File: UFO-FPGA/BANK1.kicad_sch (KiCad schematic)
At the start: 7 parts, among them U1 ICE40HX8K-BG121

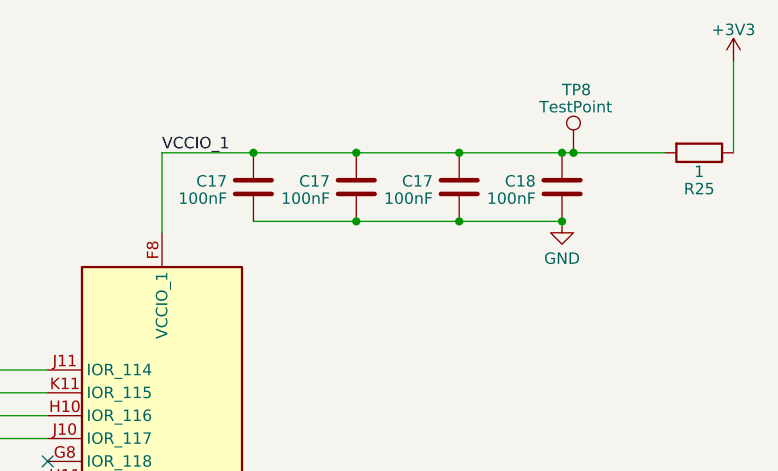
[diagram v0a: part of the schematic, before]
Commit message: PCB
many pcb changes
-started routing
-added vias
-power planes
-ground planes
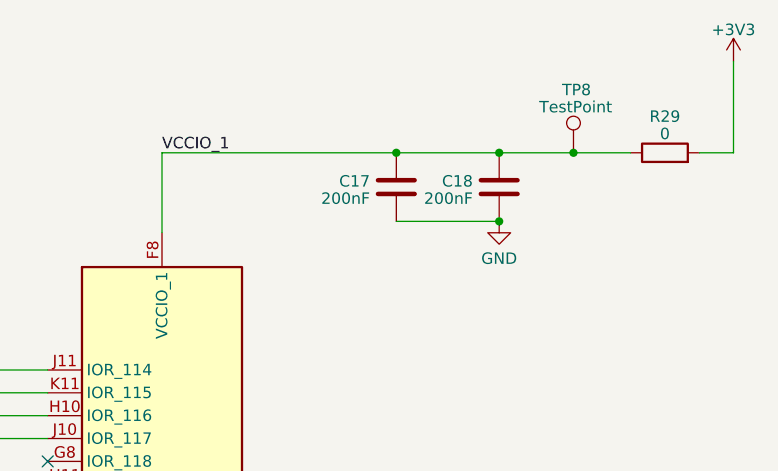
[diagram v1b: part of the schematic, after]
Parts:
- removed C17 (x3): 100nF, Capacitor_SMD:C_0805_2012Metric_Pad1.18x1.45mm_HandSolder, symbol Device:C
- removed R25: 1, Resistor_SMD:R_0805_2012Metric_Pad1.20x1.40mm_HandSolder, symbol Device:R
- added C17: 200nF, Capacitor_SMD:C_0805_2012Metric_Pad1.18x1.45mm_HandSolder, symbol Device:C
- added R29: 0, Resistor_SMD:R_0805_2012Metric_Pad1.20x1.40mm_HandSolder, symbol Device:R
- C18: value 100nF -> 200nF
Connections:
- net +3V3: now also R29.2
- net GND: now also C17.2
- net VCCIO_1: now also C17.1, R29.1
